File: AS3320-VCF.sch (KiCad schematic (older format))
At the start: 41 parts, among them J1 SIGNAL_INPUT, J2 RESONANCE_CTRL_INPUT, J3 FREQ_CTRL_INPUT, J4 SIGNAL_OUTPUT, U1 AS3320

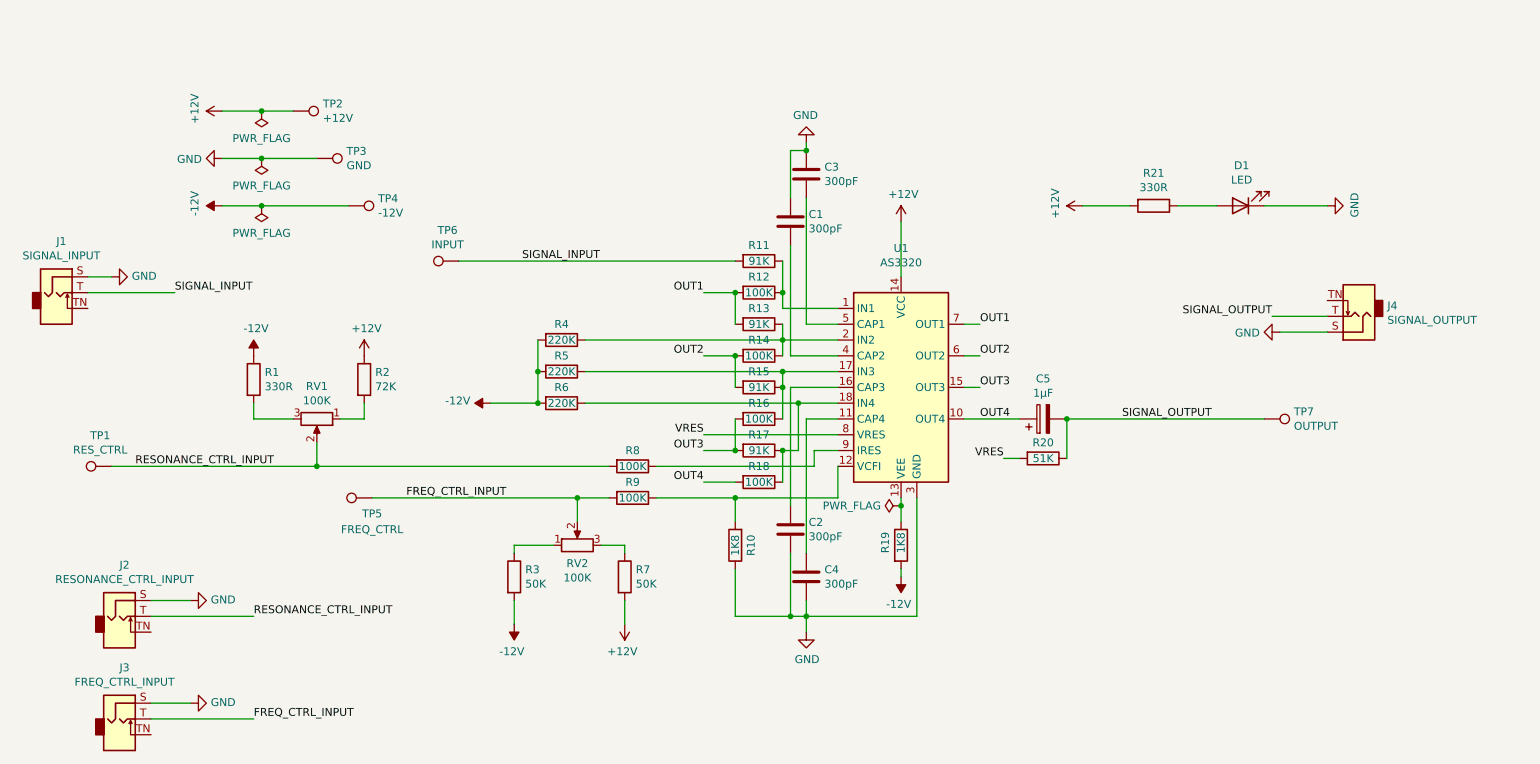
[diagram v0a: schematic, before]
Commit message: Refactor
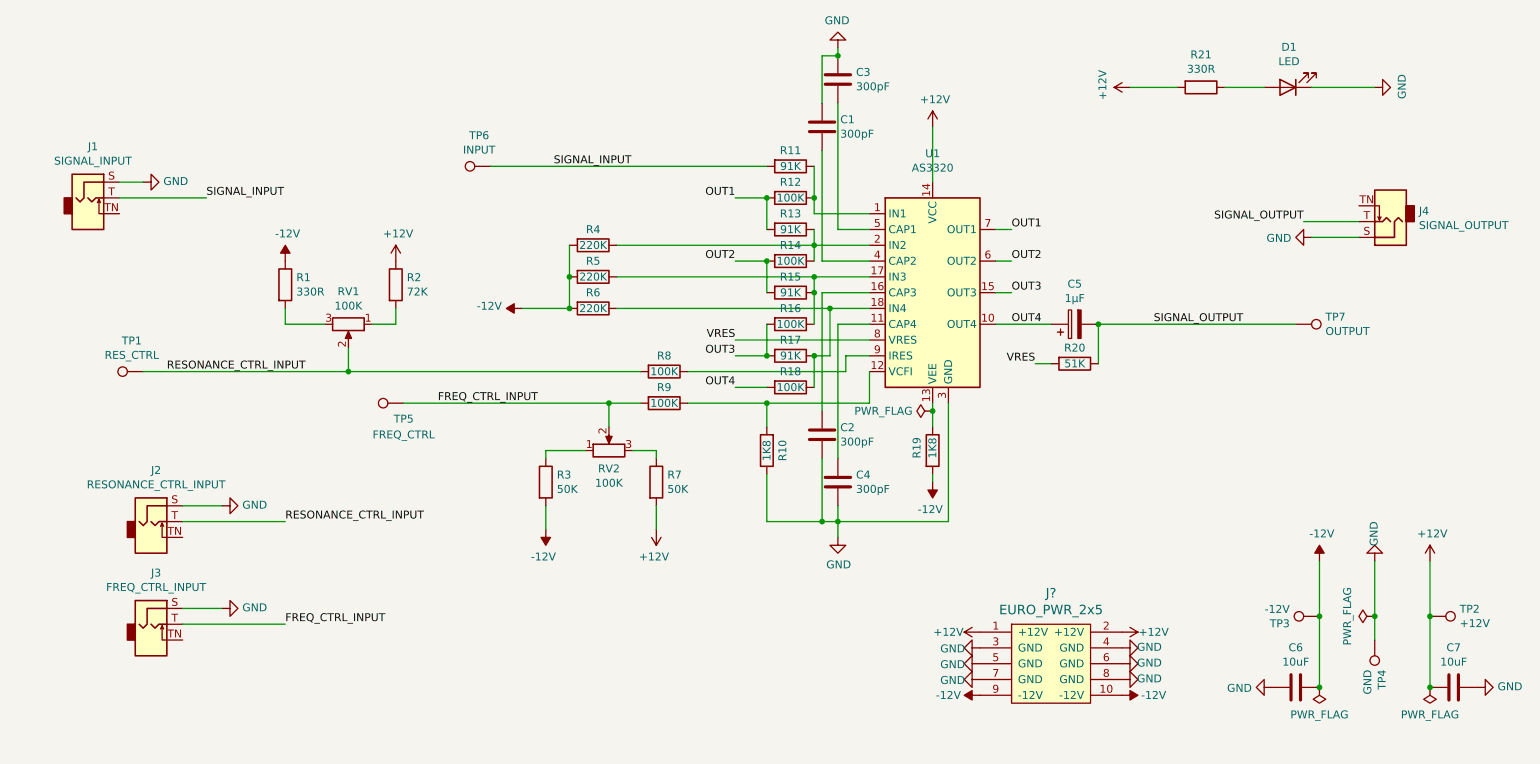
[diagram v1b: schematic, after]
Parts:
- added C6, C7: 10uF, symbol Device:C
- added J?: EURO_PWR_2x5, symbol Seattle_Synths:EURO_PWR_2x5
- TP3: value GND -> -12V
- TP4: value -12V -> GND
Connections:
- net +12V: now also C7.2, J?.1 (+12V), J?.2 (+12V)
- net -12V: now also TP3.1, C6.1, J?.10 (-12V), J?.9 (-12V); no longer TP4.1
- net GND: now also TP4.1, C6.2, C7.1, J?.3 (GND), J?.4 (GND), J?.5 (GND), J?.6 (GND), J?.7 (GND), J?.8 (GND); no longer TP3.1
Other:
- moved on the sheet: C1, C2, C3, C4, C5, D1, J1, J2, J3, J4, R1, R10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
